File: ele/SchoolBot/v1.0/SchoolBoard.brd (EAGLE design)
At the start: 95 x 60 mm, 55 parts, among them X1 M8, X2 M8, X4 POWER_IN

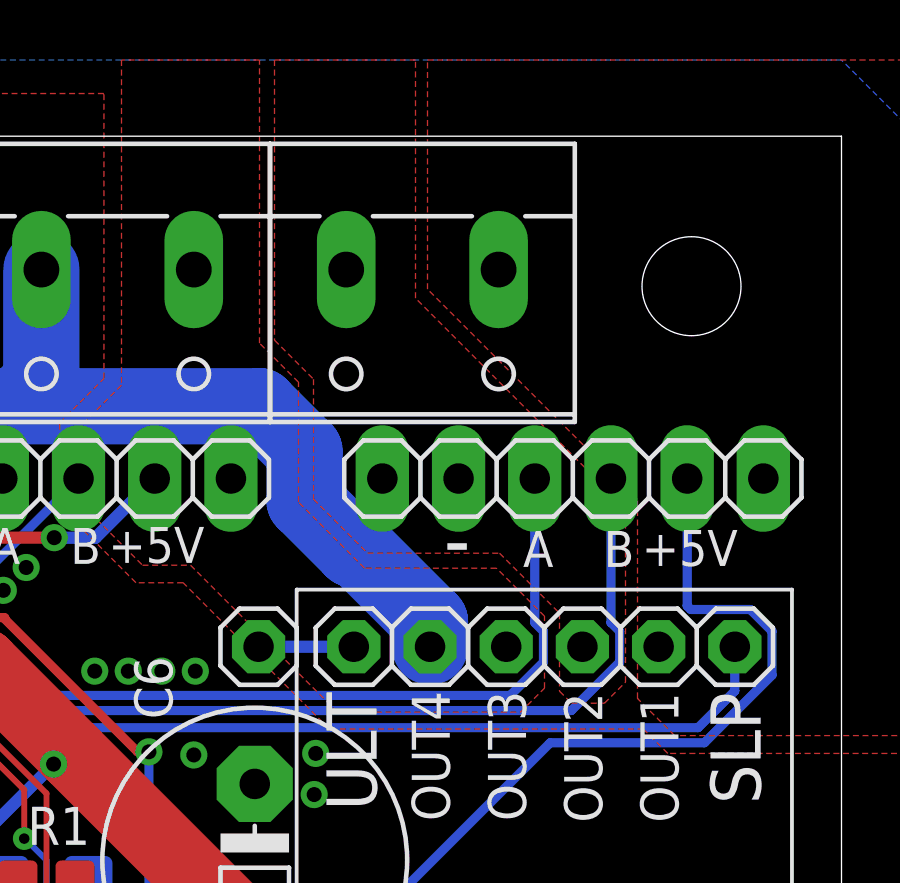
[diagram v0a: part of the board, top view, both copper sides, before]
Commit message: ir led pro encodery
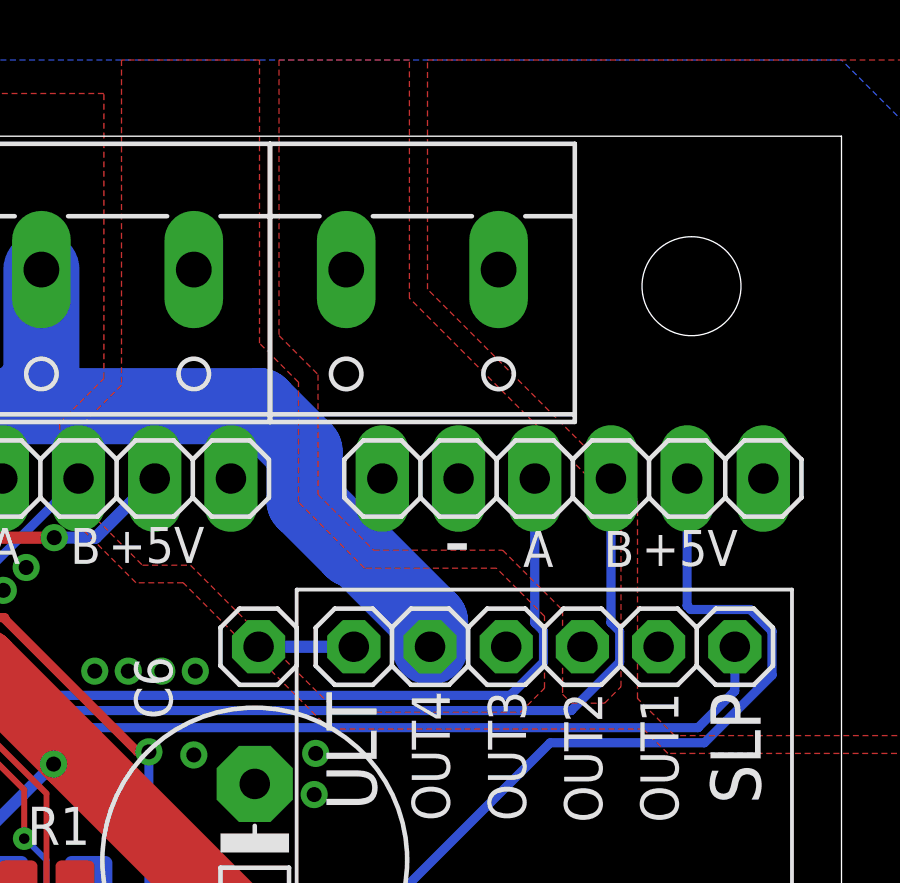
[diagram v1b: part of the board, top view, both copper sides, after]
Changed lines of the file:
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@@
 <layer number="47" name="Measures" color="7" fill="1" visible="no" active="yes"/>
 <layer number="48" name="Document" color="7" fill="1" visible="yes" active="yes"/>
-<layer number="49" name="Reference" color="7" fill="1" visible="no" active="yes"/>
+<layer number="49" name="Reference" color="7" fill="1" visible="yes" active="yes"/>
 <layer number="50" name="dxf" color="7" fill="1" visible="no" active="no"/>
 <layer number="51" name="tDocu" color="7" fill="1" visible="yes" active="yes"/>
@@
 <circle x="82.296" y="11.7348" radius="3" width="0.1524" layer="25"/>
 <rectangle x1="55.996" y1="21.9948" x2="75.996" y2="31.9948" layer="49" rot="R180"/>
-<dimension x1="0" y1="0" x2="94.996" y2="0" x3="47.498" y3="-12.7" textsize="1.778" layer="1"/>
-<dimension x1="93.98" y1="0" x2="94.0308" y2="59.8932" x3="121.9109125" y3="29.92293125" textsize="1.778" layer="1"/>
+<dimension x1="0" y1="0" x2="94.996" y2="0" x3="47.498" y3="-7.62" textsize="1.778" layer="49"/>
+<dimension x1="93.98" y1="0" x2="94.0308" y2="59.8932" x3="102.15661875" y3="29.939684375" textsize="1.778" layer="49"/>
 <text x="15.0368" y="23.622" size="1.2" layer="25" rot="R90">+3V</text>
 <text x="8.2296" y="12.3952" size="2" layer="25" rot="R180">GND</text>
@@
 <contactref element="X1" pad="2"/>
 <contactref element="JP12" pad="1"/>
-<polygon width="0.2" layer="1" thermals="no">
-<vertex x="87.796" y="41.7948"/>
-<vertex x="87.796" y="47.5948"/>
-<vertex x="80.796" y="54.5948"/>
-<vertex x="80.796" y="62.5348"/>
-<vertex x="76.096" y="62.5348"/>
-<vertex x="76.096" y="53.1948"/>
-<vertex x="77.396" y="51.8948"/>
-<vertex x="77.396" y="47.8948"/>
-<vertex x="79.196" y="46.0948"/>
-<vertex x="83.596" y="46.0948"/>
-<vertex x="85.596" y="44.0948"/>
-<vertex x="85.596" y="41.4948"/>
+<polygon width="0.5" layer="1">
+<vertex x="87.6436" y="41.6424"/>
+<vertex x="87.6436" y="47.544"/>
+<vertex x="80.5928" y="54.5948"/>
+<vertex x="80.5928" y="62.5348"/>
+<vertex x="76.2484" y="62.5348"/>
+<vertex x="76.2484" y="53.3472"/>
+<vertex x="77.5484" y="52.0472"/>
+<vertex x="77.5484" y="48.0472"/>
+<vertex x="79.3992" y="46.1964"/>
+<vertex x="83.6976" y="46.1964"/>
+<vertex x="85.6976" y="44.1964"/>
+<vertex x="85.6976" y="41.3932"/>
 <vertex x="85.996" y="41.0948"/>
 <vertex x="87.096" y="41.0948"/>
